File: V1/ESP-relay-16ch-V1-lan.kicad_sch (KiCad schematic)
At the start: 27 parts, among them J3 ETHERNET, U3 LAN8710A

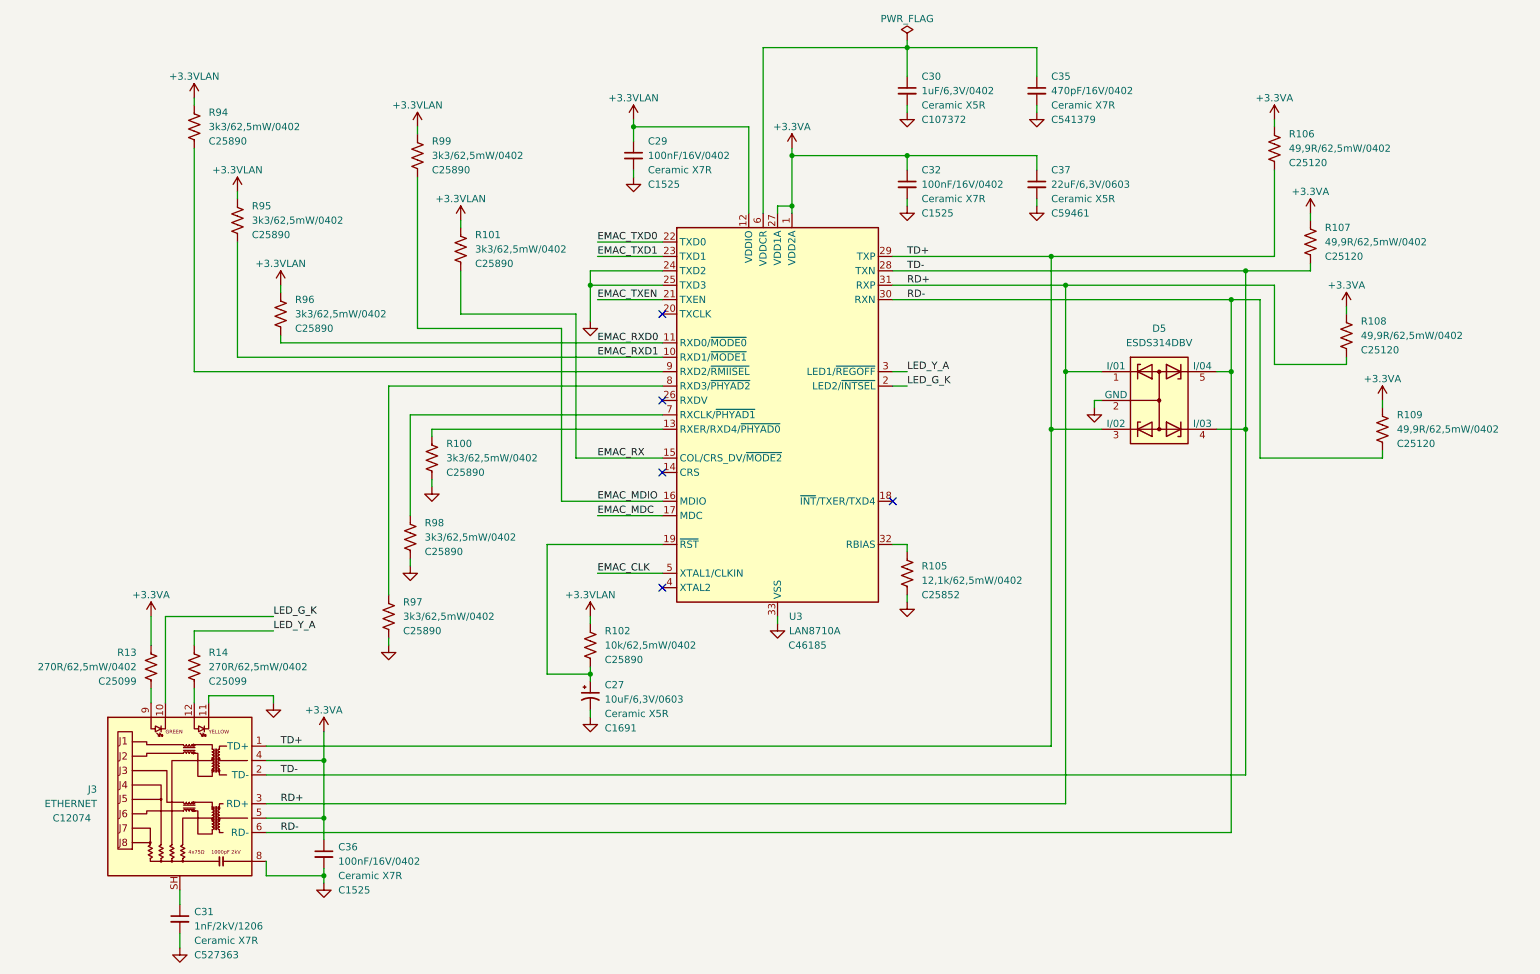
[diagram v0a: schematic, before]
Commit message: Dev updates
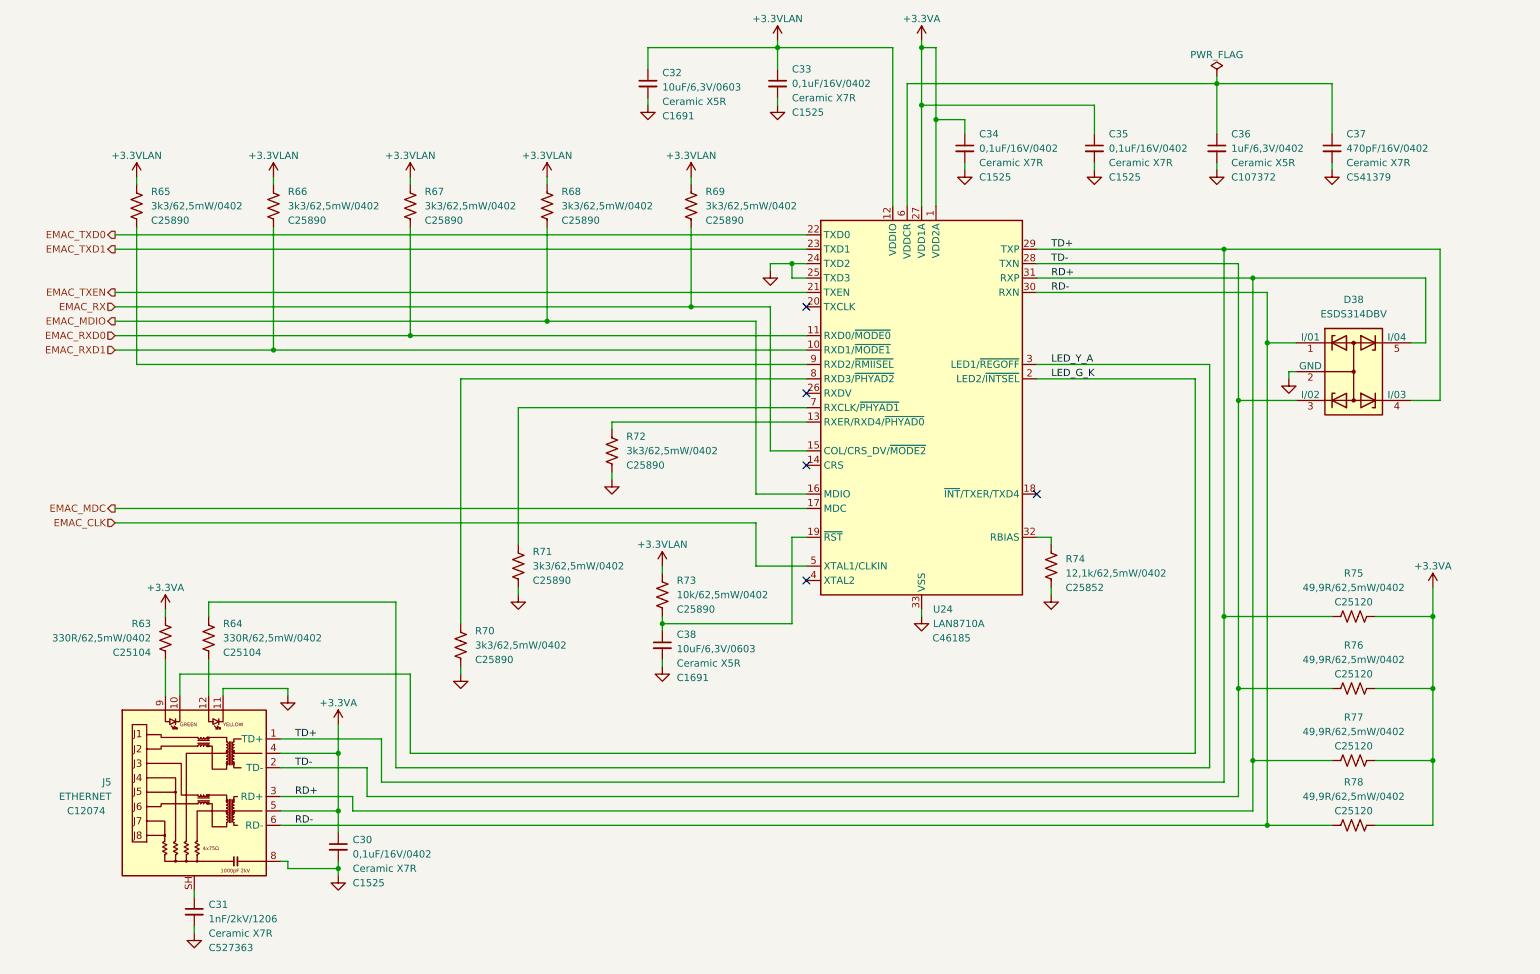
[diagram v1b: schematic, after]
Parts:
- removed C37: 22uF/6,3V/0603, Tales:C_0805_2012Metric, symbol Device:C_Small
- removed R106, R107, R108: 49,9R/62,5mW/0402, Tales:R_0402_1005Metric, symbol Device:R_US
- added C32: 10uF/6,3V/0603, Tales:C_0603_1608Metric, symbol Device:C_Small
- added C35: 0,1uF/16V/0402, Tales:C_0402_1005Metric, symbol Device:C_Small
- added R75, R76, R77: 49,9R/62,5mW/0402, Tales:R_0402_1005Metric, symbol Device:R_US
- C30: renamed from C36; value 100nF/16V/0402 -> 0,1uF/16V/0402
- C33: renamed from C29; value 100nF/16V/0402 -> 0,1uF/16V/0402
- C34: renamed from C32; value 100nF/16V/0402 -> 0,1uF/16V/0402
- C38: renamed from C27; symbol Device:C_Polarized_Small_US -> Device:C_Small
- D38: renamed from D5; Case (none) -> SOT-23-5; JLCPCB BOM (none) -> 1; LCSC Part # (none) -> C1847859; Mfr (none) -> Texas Instruments; Mfr PN (none) -> ESDS314DBVR; Vendor PN (none) -> C1847859
- R63: renamed from R13; value 270R/62,5mW/0402 -> 330R/62,5mW/0402; LCSC Part # C25099 -> C25104; Mfr PN 0402WGF2700TCE -> 0402WGF3300TCE; Vendor PN C25099 -> C25104
- R64: renamed from R14; value 270R/62,5mW/0402 -> 330R/62,5mW/0402; LCSC Part # C25099 -> C25104; Mfr PN 0402WGF2700TCE -> 0402WGF3300TCE; Vendor PN C25099 -> C25104
- U24: renamed from U3; footprint Package_DFN_QFN:QFN-32-1EP_5x5mm_P0.5mm_EP3.3x3.3mm_ThermalVias -> Tales:QFN-32-1EP_5x5mm_P0.5mm_EP3.3x3.3mm_ThermalVias
- renumbered C30 to C36, C35 to C37, J3 to J5, R94 to R65, R95 to R66, R96 to R67, R99 to R68, R101 to R69, R97 to R70, R98 to R71, R100 to R72, R102 to R73, R105 to R74, R109 to R78
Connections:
- net +3.3VA: now also R78.2, C35.1, R75.2, R76.2, R77.2; no longer R78.1
- net +3.3VLAN: now also C32.1
- net GND: now also C32.2, C35.2
- net RD+: now also D38.5 (I/04), R77.1; no longer D38.1 (I/01)
- net RD-: now also D38.1 (I/01), R78.1; no longer D38.5 (I/04), R78.2
- net TD+: now also D38.4 (I/03), R75.1; no longer D38.3 (I/02)
- net TD-: now also D38.3 (I/02), R76.1; no longer D38.4 (I/03)
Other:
- title: (none) -> ESP 16x 24VDC Input 16x External Relay Output Module
- moved on the sheet: C30, C31, C33, C34, C36, C37, D38, J5, R63, R64, R65, R66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
